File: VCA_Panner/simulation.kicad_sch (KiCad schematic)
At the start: 38 parts, among them U4 TL074, U5 TL074

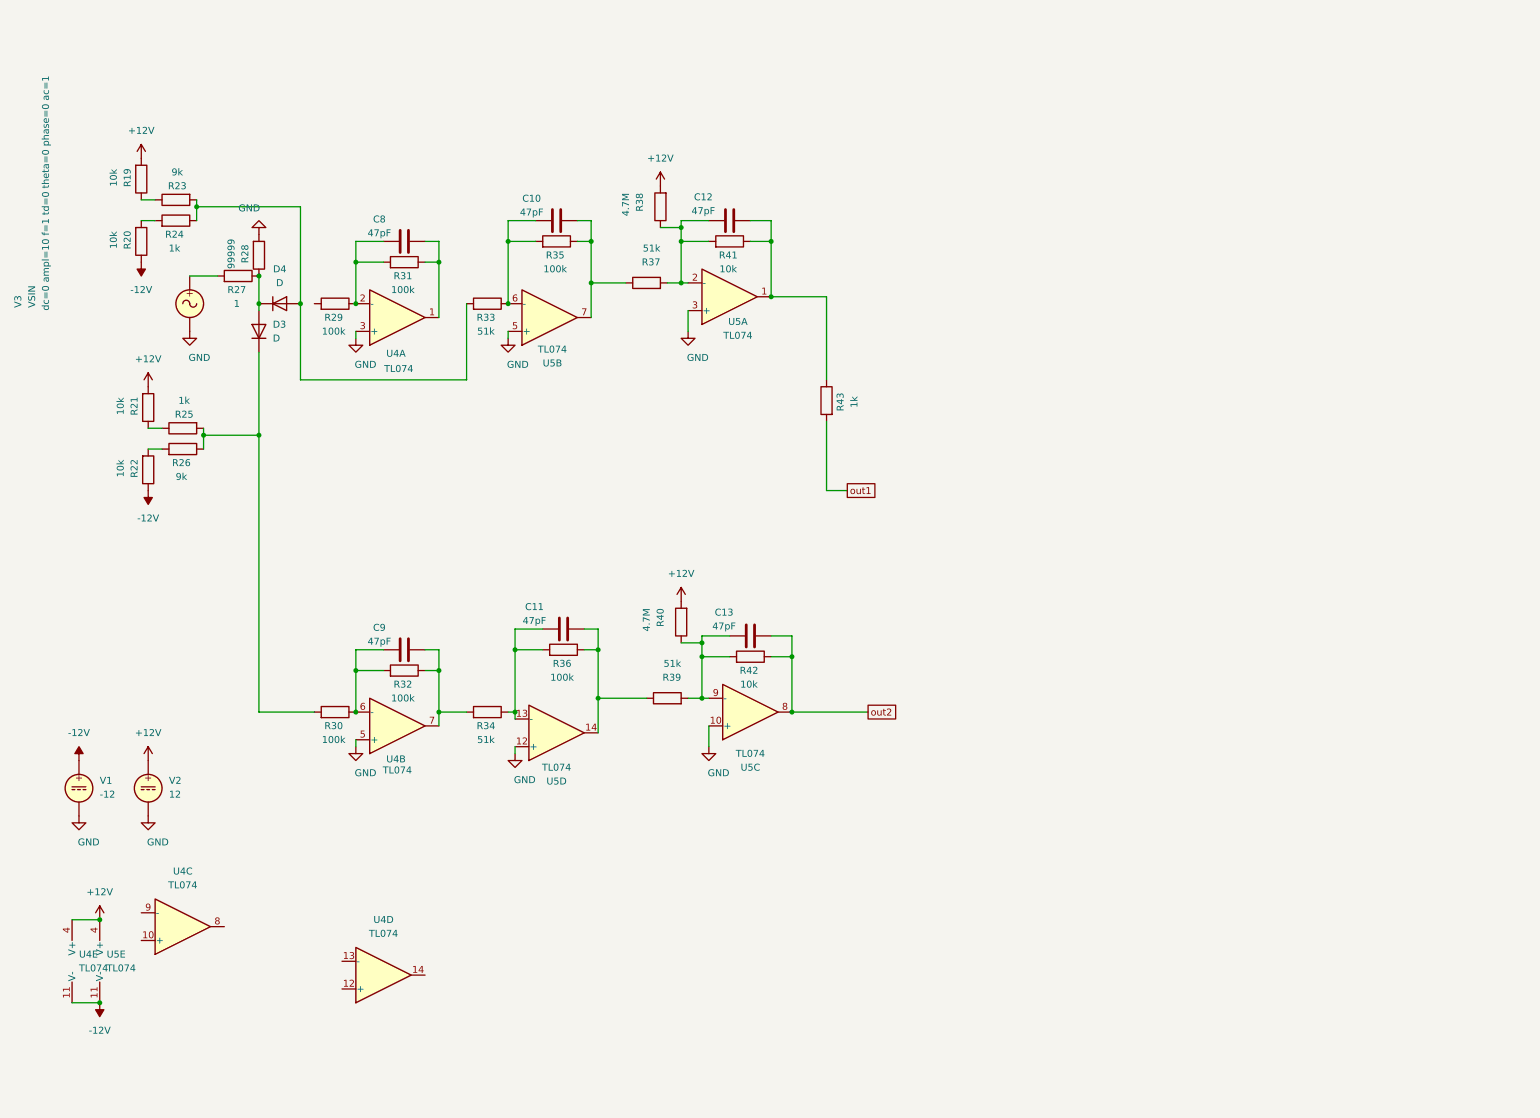
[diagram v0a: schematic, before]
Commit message: almost working
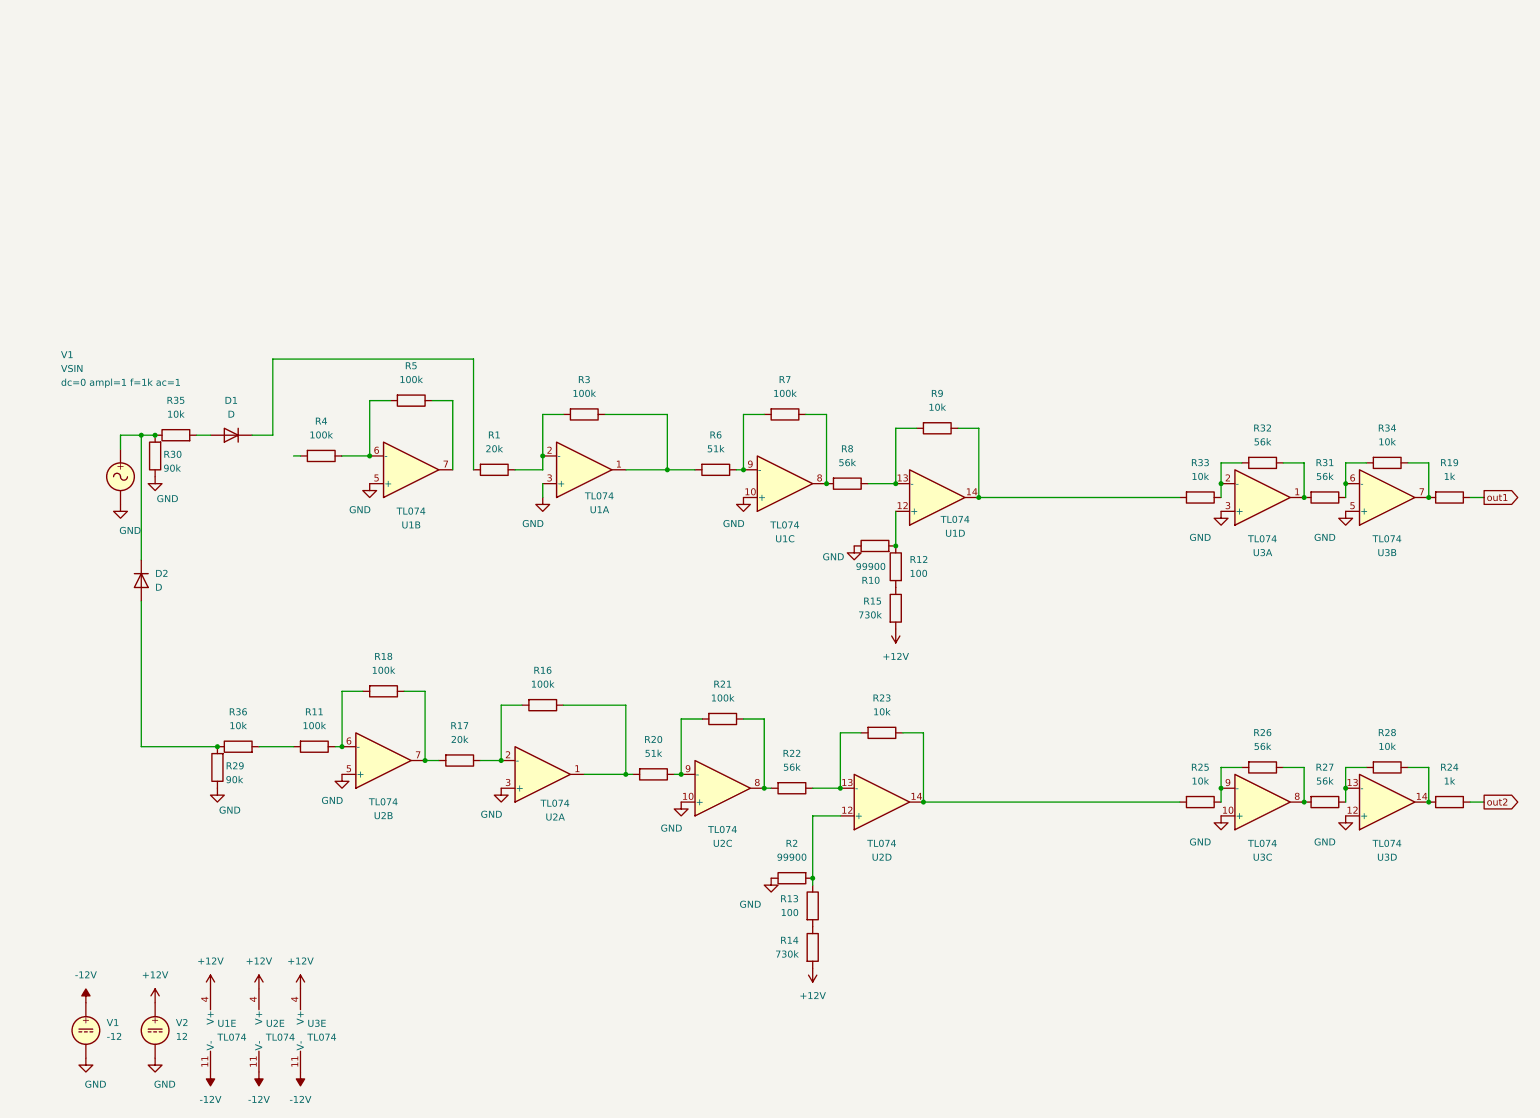
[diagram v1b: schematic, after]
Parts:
- removed C10, C11, C12, C13, C8, C9: 47pF, symbol Device:C
- removed D3, D4: D, symbol Device:D
- removed R37, R39: 51k, symbol Device:R
- removed R38, R40: 4.7M, symbol Device:R
- removed R41, R42: 10k, symbol Device:R
- removed R43: 1k, symbol Device:R
- removed U4, U5: TL074, symbol Amplifier_Operational:TL074
- removed V3: VSIN, symbol Simulation_SPICE:VSIN
- added D1, D2: D, symbol Device:D
- added R1, R17: 20k, symbol Device:R
- added R10, R2: 99900, symbol Device:R
- added R11, R16, R18, R3, R4, R5, R7: 100k, symbol Device:R
- added R12, R13: 100, symbol Device:R
- added R14, R15: 730k, symbol Device:R
- added R6: 51k, symbol Device:R
- added R8: 56k, symbol Device:R
- added R9: 10k, symbol Device:R
- added U1, U2, U3: TL074, symbol Amplifier_Operational:TL074
- added V1: VSIN, symbol Simulation_SPICE:VSIN
- R19: value 10k -> 1k
- R20: value 10k -> 51k
- R21: value 10k -> 100k
- R22: value 10k -> 56k
- R23: value 9k -> 10k
- R25: value 1k -> 10k
- R26: value 9k -> 56k
- R27: value 1 -> 56k
- R28: value 99999 -> 10k
- R29, R30: value 100k -> 90k
- R31, R32: value 100k -> 56k
- R33, R34: value 51k -> 10k
- R35, R36: value 100k -> 10k
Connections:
- net +12V: now also R14.2, R15.2, U1.4 (V+), U2.4 (V+), U3.4 (V+); no longer R19.2, R21.2
- net -12V: now also U1.11 (V-), U2.11 (V-), U3.11 (V-); no longer R20.1, R22.1
- net GND: now also R29.1, R30.1, R10.1, R2.1, U1.10 (+), U1.3 (+), U1.5 (+), U2.10 (+), U2.3 (+), U2.5 (+), U3.10 (+), U3.12 (+), U3.3 (+), U3.5 (+), V1.2; no longer R28.2
- net out1: now also R19.1
- net out2: now also R24.1
- net at R31.1: now also R34.2, U3.6 (-)
- net at R31.2: now also R32.1, U3.1; no longer R29.1
- net at R32.2: now also R33.1, U3.2 (-); no longer R30.1
- net at R23.1: now also R25.2, U2.14; no longer R19.1
- net at R20.2: now also R16.1, U2.1; no longer R24.2
- net at R25.1: now also R26.2, U3.9 (-); no longer R21.1
- net at R27.2: now also R26.1, U3.8
- net at R29.2: now also R36.1, D2.2 (A)
- net at R35.1: now also R30.2, D2.1 (K), V1.1
- net at R34.1: now also R19.2, U3.7; no longer R36.2
- net at R22.2: now also R21.1, U2.8; no longer R26.2
- net at R35.2: now also D1.2 (A); no longer R33.1
- net at R27.1: now also R28.2, U3.13 (-); no longer R28.1
- new net: R5.1, U1.7
- new net: R4.1, R5.2, U1.6 (-)
- new net: R20.1, R21.2, U2.9 (-)
- new net: R7.1, R8.2, U1.8
- new net: R6.1, R7.2, U1.9 (-)
- new net: R10.2, R12.1, U1.12 (+)
- new net: R12.2, R15.1
- new net: R13.1, R2.2, U2.12 (+)
- new net: R13.2, R14.1
- new net: R16.2, R17.1, U2.2 (-)
- new net: R24.2, R28.1, U3.14
- new net: R22.1, R23.2, U2.13 (-)
- new net: R3.1, R6.2, U1.1
- new net: R1.1, R3.2, U1.2 (-)
- new net: D1.1 (K), R1.2
- new net: R33.2, R9.1, U1.14
- new net: R8.1, R9.2, U1.13 (-)
- new net: R11.1, R18.2, U2.6 (-)
- new net: R17.2, R18.1, U2.7
- new net: R11.2, R36.2
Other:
- moved on the sheet: V1, V2
